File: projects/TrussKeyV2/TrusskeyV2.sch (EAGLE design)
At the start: 44 parts, among them J1 M20-9980346, J2 MOLEX_503480-0600MOLEX_503480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, J3 10104111-0001LF, J4 5-146280-1, J5 5-146280-1, J6 MOLEX_503480-0600MOLEX_503480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, J7 5-146280-1, Q1 ABM-16MHZ, SW1 LS12T2-T, SW2 EVQ11U09K, SW3 ESE31L11T, U2 TPS62200, U3 LC709203, U5 MCP73831T-2ACI/OT, X1 CON-1PIN, X3 CON-1PIN

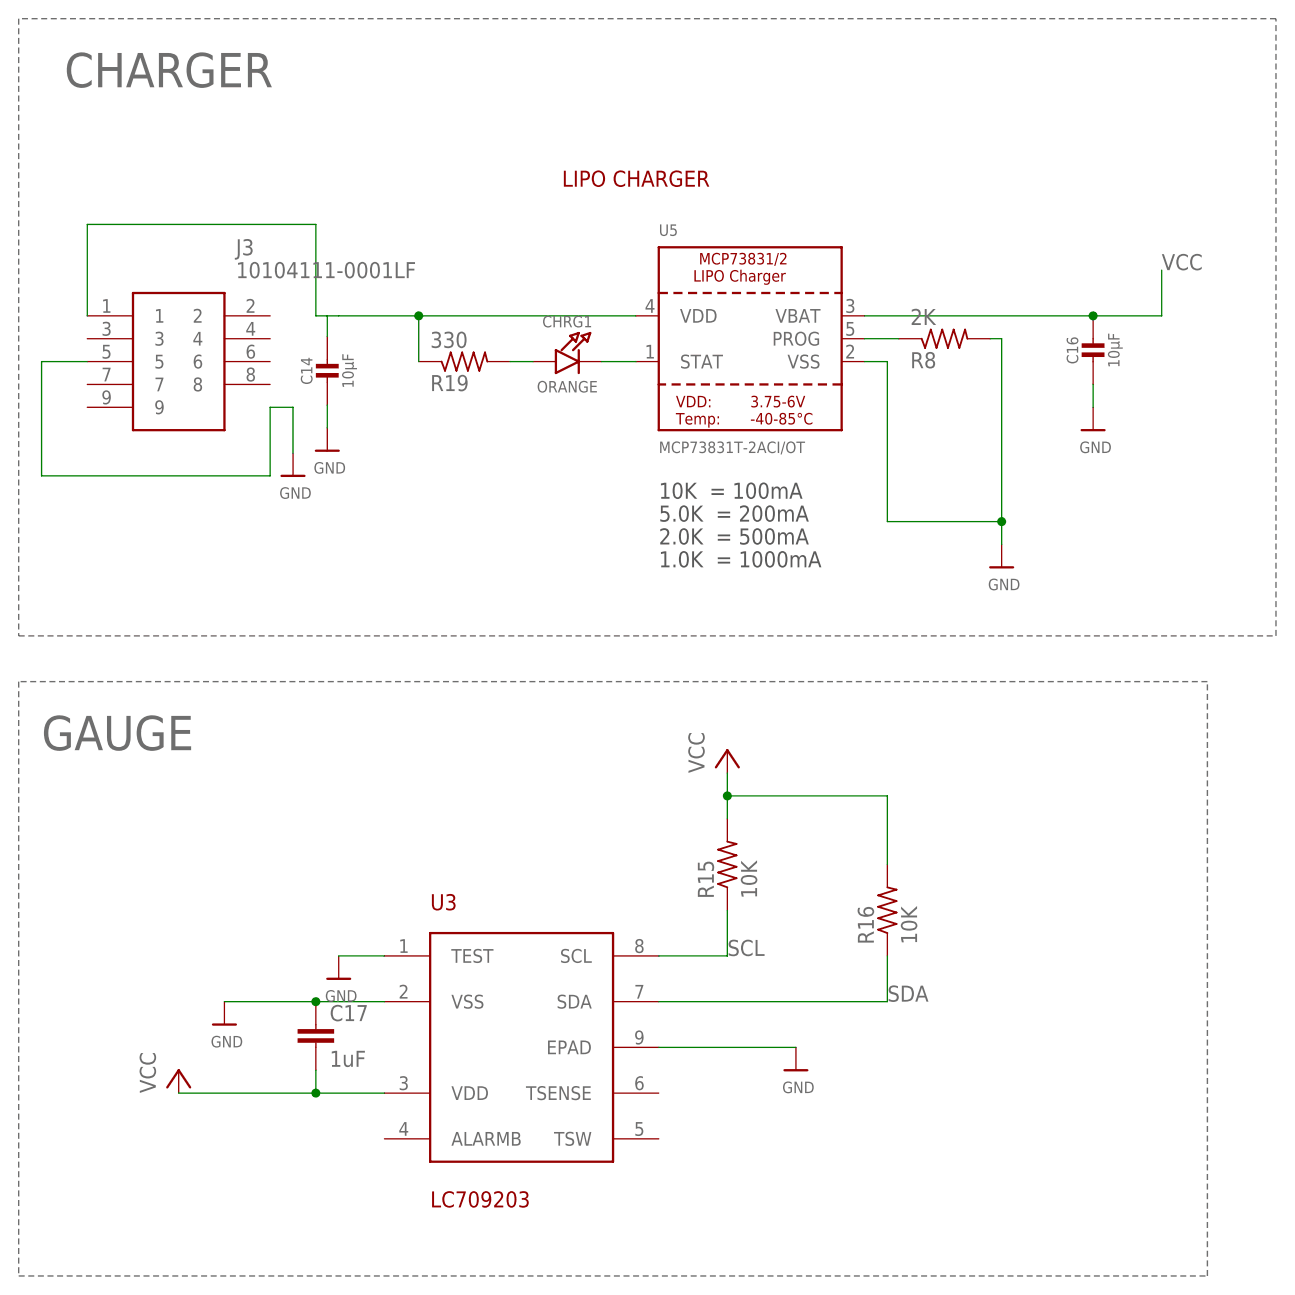
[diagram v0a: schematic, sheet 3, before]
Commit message: GasGauge
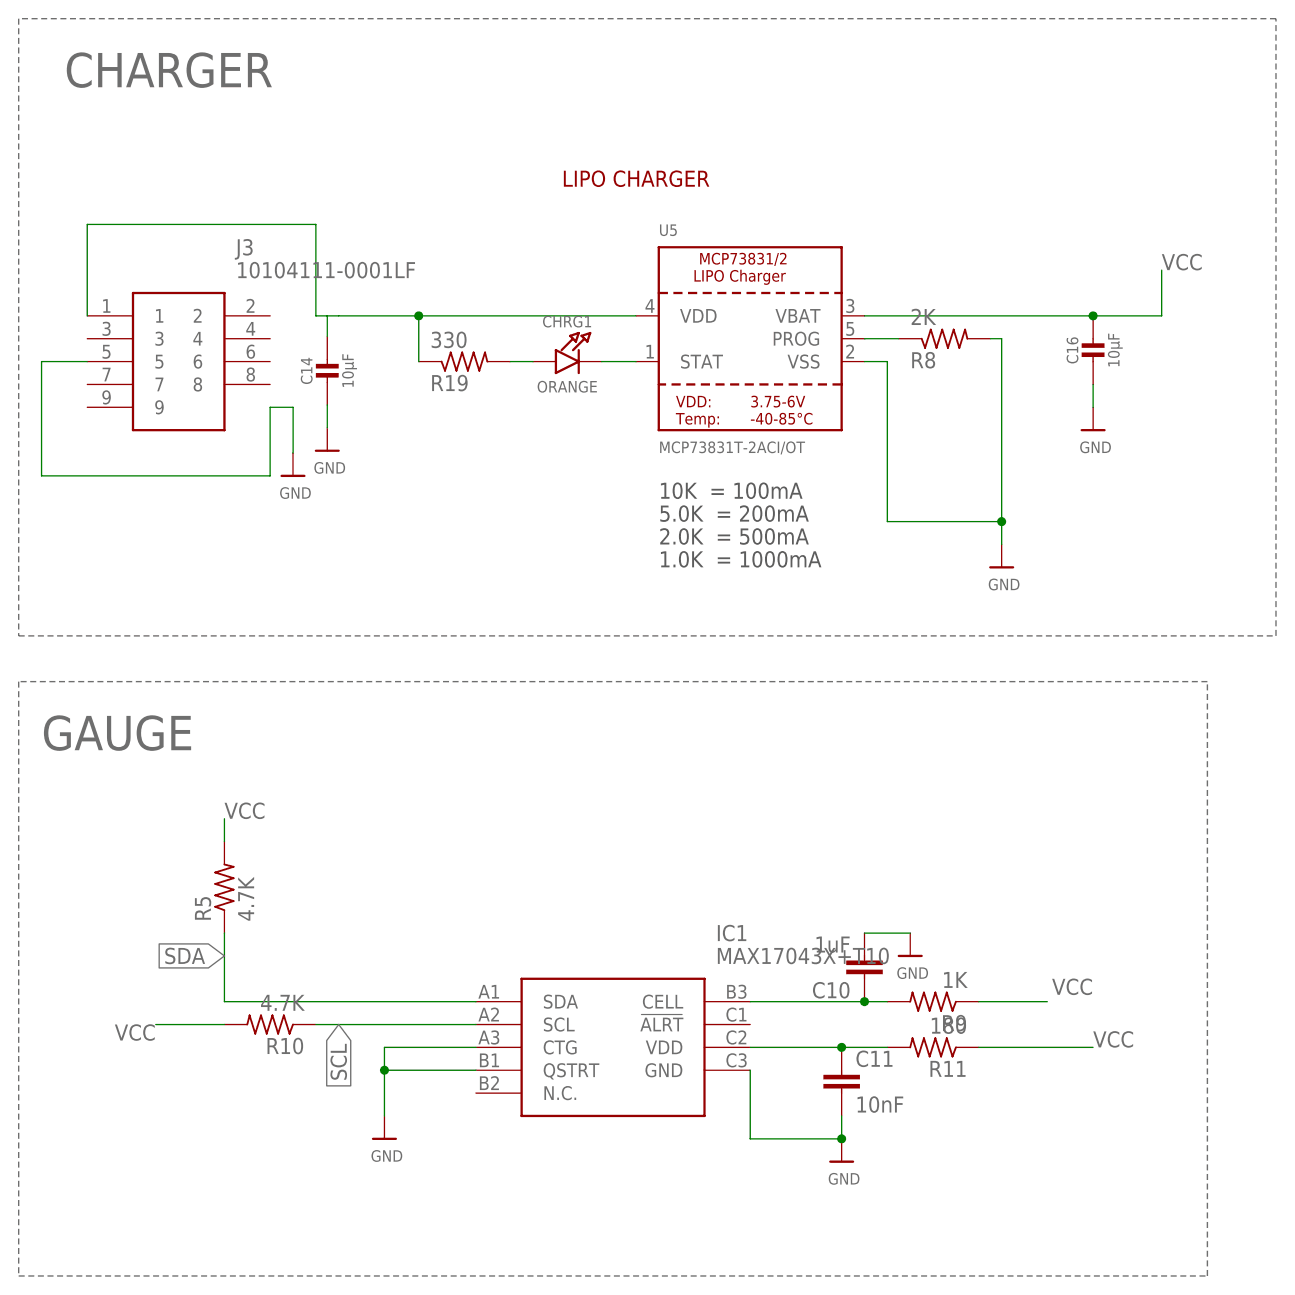
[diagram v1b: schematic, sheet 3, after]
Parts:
- removed C17: 1uF, rcl:C-EUC0603
- removed R15, R16: 10K, resistor:R-US_R0402
- removed U3: LC709203, NewPart:LC709203
- added C10: 1uF, rcl:C-EUC0603
- added C11: 10nF, rcl:C-EUC0603
- added IC1: MAX17043X+T10, SamacSys_Parts:MAX17043X+T10
- added R10, R5: 4.7K, resistor:R-US_R0402
- added R11: 180, resistor:R-US_R0402
- added R9: 1K, resistor:R-US_R0402
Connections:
- new net N$10: C10.1, IC1.CELL, R9.2
- new net N$9: C11.1, IC1.VDD, R11.2
- net GND: now also C10.2, C11.2, IC1.CTG, IC1.GND, IC1.QSTRT; no longer C17.1, U3.EPAD, U3.TEST, U3.VSS
- net SCL: now also IC1.SCL, R10.1; no longer R15.1, U3.SCL
- net SDA: now also IC1.SDA, R5.1; no longer R16.1, U3.SDA
- net VCC: now also R10.2, R11.1, R5.2, R9.1; no longer C17.2, R15.2, R16.2, U3.VDD
